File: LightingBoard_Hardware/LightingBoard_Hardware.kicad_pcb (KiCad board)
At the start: 2 copper layers, 61 x 108.8 mm, 22 parts, among them U1 LDD-1500L, U2 LDD-1500L, U3 TM4C129E_Launchpad, U4 +5V OKI

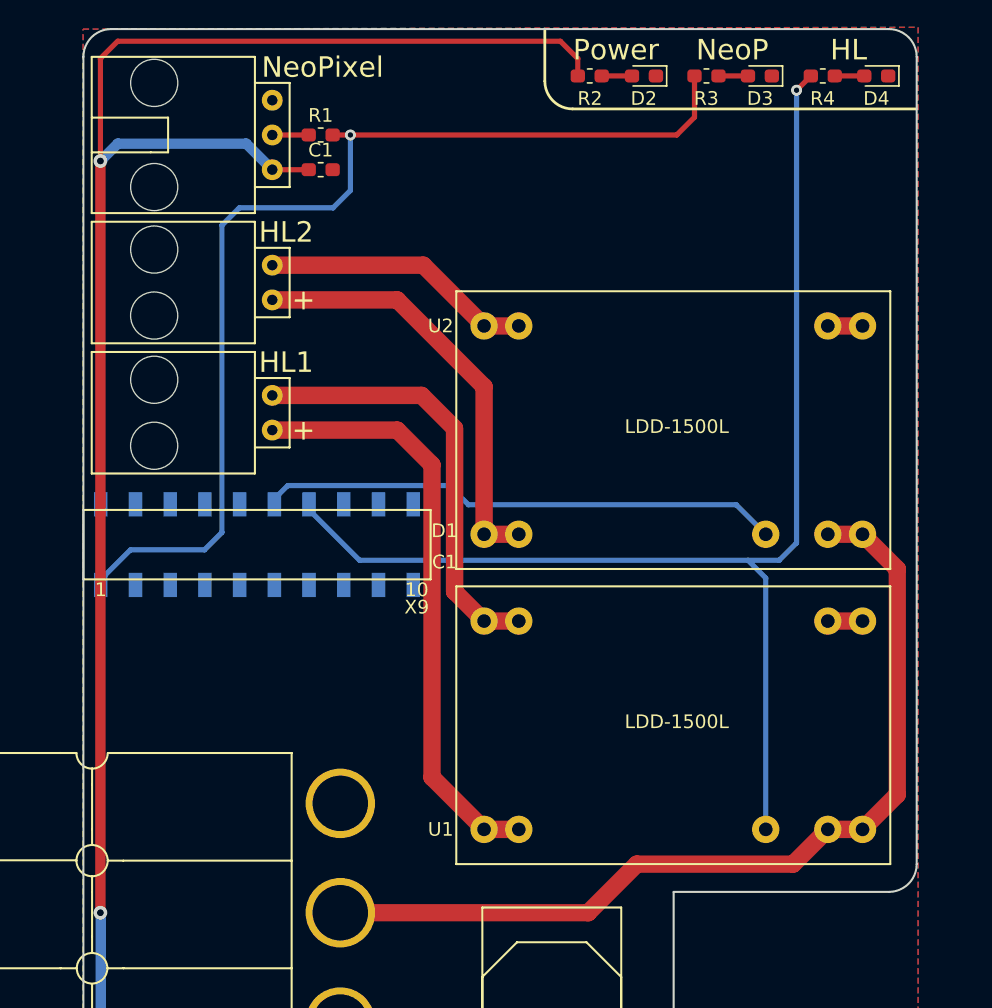
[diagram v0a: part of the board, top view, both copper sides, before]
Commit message: Final Board
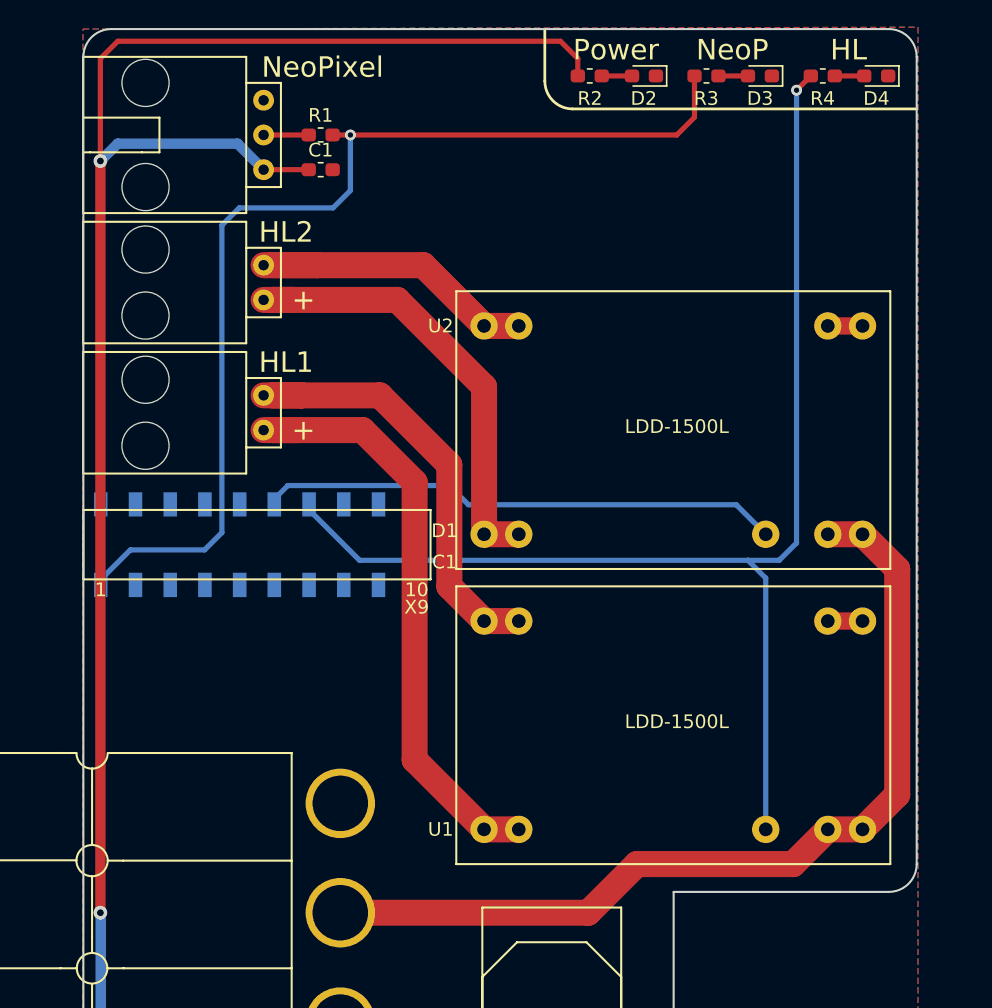
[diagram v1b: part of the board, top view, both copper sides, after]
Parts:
- moved Conn2 0.64 mm to (114.7, 68.2)
- moved Conn3 0.64 mm to (114.7, 58.7)
- moved Conn4 0.64 mm to (114.7, 47.9)
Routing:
- net /Headlight_V2-: track 19.9 -> 23.8 mm
- net /Headlight_V2+: track 31.5 -> 33.6 mm
- net /Headlight_V1+: track 43.5 -> 44.6 mm
- net /Headlight_V1-: track 31.9 -> 32.9 mm
- net Net-(Conn4-Pad2): track 2.67 -> 3.30 mm
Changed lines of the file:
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@@
     (thickness 1.6)
     (drawings 30)
-    (tracks 91)
+    (tracks 99)
     (zones 0)
     (modules 22)
@@
   )
   (setup
-    (last_trace_width 0.25)
+    (last_trace_width 1.905)
     (user_trace_width 0.0381)
     (user_trace_width 0.03998)
@@
     (user_trace_width 0.762)
     (user_trace_width 1.27)
+    (user_trace_width 1.905)
     (trace_clearance 0.2)
     (zone_clearance 0.508)
@@
     (solder_mask_min_width 0.25)
     (aux_axis_origin 0 0)
-    (visible_elements 7FFFFFFF)
+    (visible_elements 7FFFEFFF)
     (pcbplotparams
       (layerselection 0x010fc_ffffffff)
@@
   )
   (module MRDT_Connectors:MOLEX_SL_02_Horizontal (layer F.Cu)
-    (at 115.316 68.199 90)
+    (at 114.681 68.199 90)
     (fp_text reference Conn2 (at 0 2.54 90) (layer F.SilkS) hide
       (effects (font (size 1 1) (thickness 0.15)))
@@
   )
   (module MRDT_Connectors:MOLEX_SL_02_Horizontal (layer F.Cu)
-    (at 115.316 58.674 90)
+    (at 114.681 58.674 90)
     (fp_text reference Conn3 (at 0 2.54 90) (layer F.SilkS) hide
       (effects (font (size 1 1) (thickness 0.15)))
@@
   )
   (module MRDT_Connectors:MOLEX_SL_03_Horizontal (layer F.Cu)
-    (at 115.316 47.879 90)
+    (at 114.681 47.879 90)
     (fp_text reference Conn4 (at -1.27 2.54 90) (layer F.SilkS) hide
       (effects (font (size 1 1) (thickness 0.15)))
@@
   (gr_arc (start 101.4984 136.271) (end 101.4984 138.303) (angle -180) (layer Edge.Cuts) (width 0.15))
   (segment (start 133.223 119.634) (end 133.223 123.317) (width 0.381) (layer F.Cu) (net 1))
-  (segment (start 117.983 50.419) (end 115.316 50.419) (width 0.381) (layer F.Cu) (net 1))
   (segment (start 102.768001 118.477301) (end 102.768001 118.083601) (width 0.762) (layer B.Cu) (net 1))
   (segment (start 102.768001 118.477301) (end 103.9247 119.634) (width 0.762) (layer B.Cu) (net 1))
@@
   (via (at 102.743 49.784) (size 1) (drill 0.5) (layers F.Cu B.Cu) (net 1))
   (segment (start 102.743 49.784) (end 104.013 48.514) (width 0.762) (layer B.Cu) (net 1))
-  (segment (start 115.316 50.419) (end 113.411 48.514) (width 0.762) (layer B.Cu) (net 1))
-  (segment (start 113.411 48.514) (end 104.013 48.514) (width 0.762) (layer B.Cu) (net 1))
+  (segment (start 114.681 50.419) (end 112.776 48.514) (width 0.762) (layer B.Cu) (net 1))
+  (segment (start 112.776 48.514) (end 104.013 48.514) (width 0.762) (layer B.Cu) (net 1))
+  (segment (start 117.983 50.419) (end 114.681 50.419) (width 0.381) (layer F.Cu) (net 1))
   (segment (start 158.496 83.439) (end 155.956 83.439) (width 1.27) (layer F.Cu) (net 2))
   (segment (start 158.496 61.849) (end 155.956 61.849) (width 1.27) (layer F.Cu) (net 2))
@@
   (segment (start 135.763 112.776) (end 138.303 115.316) (width 0.762) (layer F.Cu) (net 3))
   (segment (start 138.303 115.316) (end 138.303 119.634) (width 0.762) (layer F.Cu) (net 3))
-  (segment (start 158.496 98.679) (end 155.956 98.679) (width 1.27) (layer F.Cu) (net 4))
-  (segment (start 158.496 77.089) (end 155.956 77.089) (width 1.27) (layer F.Cu) (net 4))
-  (segment (start 120.2944 104.776) (end 138.429 104.776) (width 1.27) (layer F.Cu) (net 4))
-  (segment (start 138.429 104.776) (end 141.986 101.219) (width 1.27) (layer F.Cu) (net 4))
-  (segment (start 141.986 101.219) (end 153.416 101.219) (width 1.27) (layer F.Cu) (net 4))
-  (segment (start 153.416 101.219) (end 155.956 98.679) (width 1.27) (layer F.Cu) (net 4))
-  (segment (start 158.496 98.679) (end 161.036 96.139) (width 1.27) (layer F.Cu) (net 4))
-  (segment (start 161.036 96.139) (end 161.036 79.629) (width 1.27) (layer F.Cu) (net 4))
-  (segment (start 161.036 79.629) (end 158.496 77.089) (width 1.27) (layer F.Cu) (net 4))
-  (segment (start 133.35 98.679) (end 130.81 98.679) (width 1.27) (layer F.Cu) (net 5))
-  (segment (start 130.81 98.679) (end 127 94.869) (width 1.27) (layer F.Cu) (net 5))
-  (segment (start 127 94.869) (end 127 72.009) (width 1.27) (layer F.Cu) (net 5))
-  (segment (start 127 72.009) (end 124.46 69.469) (width 1.27) (layer F.Cu) (net 5))
-  (segment (start 124.46 69.469) (end 115.316 69.469) (width 1.27) (layer F.Cu) (net 5))
-  (segment (start 133.35 83.439) (end 130.81 83.439) (width 1.27) (layer F.Cu) (net 6))
-  (segment (start 126.238 66.929) (end 115.316 66.929) (width 1.27) (layer F.Cu) (net 6))
-  (segment (start 128.651 69.342) (end 126.238 66.929) (width 1.27) (layer F.Cu) (net 6))
-  (segment (start 130.81 83.439) (end 128.651 81.28) (width 1.27) (layer F.Cu) (net 6))
-  (segment (start 128.651 81.28) (end 128.651 69.342) (width 1.27) (layer F.Cu) (net 6))
-  (segment (start 133.35 61.849) (end 130.81 61.849) (width 1.27) (layer F.Cu) (net 7))
-  (segment (start 130.81 61.849) (end 126.365 57.404) (width 1.27) (layer F.Cu) (net 7))
-  (segment (start 126.365 57.404) (end 115.316 57.404) (width 1.27) (layer F.Cu) (net 7))
-  (segment (start 133.35 77.089) (end 130.81 77.089) (width 1.27) (layer F.Cu) (net 8))
-  (segment (start 130.81 77.089) (end 130.81 66.294) (width 1.27) (layer F.Cu) (net 8))
-  (segment (start 130.81 66.294) (end 124.46 59.944) (width 1.27) (layer F.Cu) (net 8))
-  (segment (start 124.46 59.944) (end 115.316 59.944) (width 1.27) (layer F.Cu) (net 8))
-  (segment (start 117.983 47.879) (end 115.316 47.879) (width 0.381) (layer F.Cu) (net 9))
+  (segment (start 120.2944 104.776) (end 138.429 104.776) (width 1.905) (layer F.Cu) (net 4))
+  (segment (start 138.429 104.776) (end 141.986 101.219) (width 1.905) (layer F.Cu) (net 4))
+  (segment (start 141.986 101.219) (end 153.416 101.219) (width 1.905) (layer F.Cu) (net 4))
+  (segment (start 153.416 101.219) (end 155.956 98.679) (width 1.905) (layer F.Cu) (net 4))
+  (segment (start 155.956 98.679) (end 158.496 98.679) (width 1.905) (layer F.Cu) (net 4))
+  (segment (start 158.496 98.679) (end 161.036 96.139) (width 1.905) (layer F.Cu) (net 4))
+  (segment (start 161.036 96.139) (end 161.036 79.629) (width 1.905) (layer F.Cu) (net 4))
+  (segment (start 161.036 79.629) (end 158.496 77.089) (width 1.905) (layer F.Cu) (net 4))
+  (segment (start 158.496 77.089) (end 155.956 77.089) (width 1.905) (layer F.Cu) (net 4))
+  (segment (start 130.81 98.679) (end 125.73 93.599) (width 1.905) (layer F.Cu) (net 5))
+  (segment (start 125.73 93.599) (end 125.73 73.279) (width 1.905) (layer F.Cu) (net 5))
+  (segment (start 125.73 73.279) (end 121.92 69.469) (width 1.905) (layer F.Cu) (net 5))
+  (segment (start 130.81 98.679) (end 133.35 98.679) (width 1.905) (layer F.Cu) (net 5))
+  (segment (start 114.681 69.469) (end 117.221 69.469) (width 1.905) (layer F.Cu) (net 5))
+  (segment (start 121.92 69.469) (end 117.221 69.469) (width 1.905) (layer F.Cu) (net 5))
+  (segment (start 117.221 69.469) (end 115.316 69.469) (width 1.905) (layer F.Cu) (net 5))
+  (segment (start 130.81 83.439) (end 133.35 83.439) (width 1.905) (layer F.Cu) (net 6))
+  (segment (start 128.27 80.899) (end 130.81 83.439) (width 1.905) (layer F.Cu) (net 6))
+  (segment (start 128.27 72.009) (end 128.27 80.899) (width 1.905) (layer F.Cu) (net 6))
+  (segment (start 123.19 66.929) (end 128.27 72.009) (width 1.905) (layer F.Cu) (net 6))
+  (segment (start 114.681 66.929) (end 117.475 66.929) (width 1.905) (layer F.Cu) (net 6))
+  (segment (start 115.316 66.929) (end 117.475 66.929) (width 1.905) (layer F.Cu) (net 6))
+  (segment (start 117.475 66.929) (end 123.19 66.929) (width 1.905) (layer F.Cu) (net 6))
+  (segment (start 133.35 61.849) (end 130.81 61.849) (width 1.905) (layer F.Cu) (net 7))
+  (segment (start 130.81 61.849) (end 126.365 57.404) (width 1.905) (layer F.Cu) (net 7))
+  (segment (start 114.681 57.404) (end 118.618 57.404) (width 1.905) (layer F.Cu) (net 7))
+  (segment (start 126.365 57.404) (end 118.618 57.404) (width 1.905) (layer F.Cu) (net 7))
+  (segment (start 118.618 57.404) (end 115.316 57.404) (width 1.905) (layer F.Cu) (net 7))
+  (segment (start 133.35 77.089) (end 130.81 77.089) (width 1.905) (layer F.Cu) (net 8))
+  (segment (start 130.81 77.089) (end 130.81 66.294) (width 1.905) (layer F.Cu) (net 8))
+  (segment (start 130.81 66.294) (end 124.46 59.944) (width 1.905) (layer F.Cu) (net 8))
+  (segment (start 114.681 59.944) (end 116.84 59.944) (width 1.905) (layer F.Cu) (net 8))
+  (segment (start 124.46 59.944) (end 116.84 59.944) (width 1.905) (layer F.Cu) (net 8))
+  (segment (start 116.84 59.944) (end 115.316 59.944) (width 1.905) (layer F.Cu) (net 8))
+  (segment (start 117.983 47.879) (end 114.681 47.879) (width 0.381) (layer F.Cu) (net 9))
   (segment (start 139.418 43.561) (end 141.633 43.561) (width 0.381) (layer F.Cu) (net 10))
   (segment (start 147.955 43.561) (end 150.114 43.561) (width 0.381) (layer F.Cu) (net 11))
